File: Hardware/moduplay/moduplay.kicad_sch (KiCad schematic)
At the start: 11 parts, among them SW1 Left, SW10 Power_Switch, SW2 Up, SW3 Right, SW4 Down, SW5 X, SW6 Y, SW7 B, SW8 A, SW9 Menu

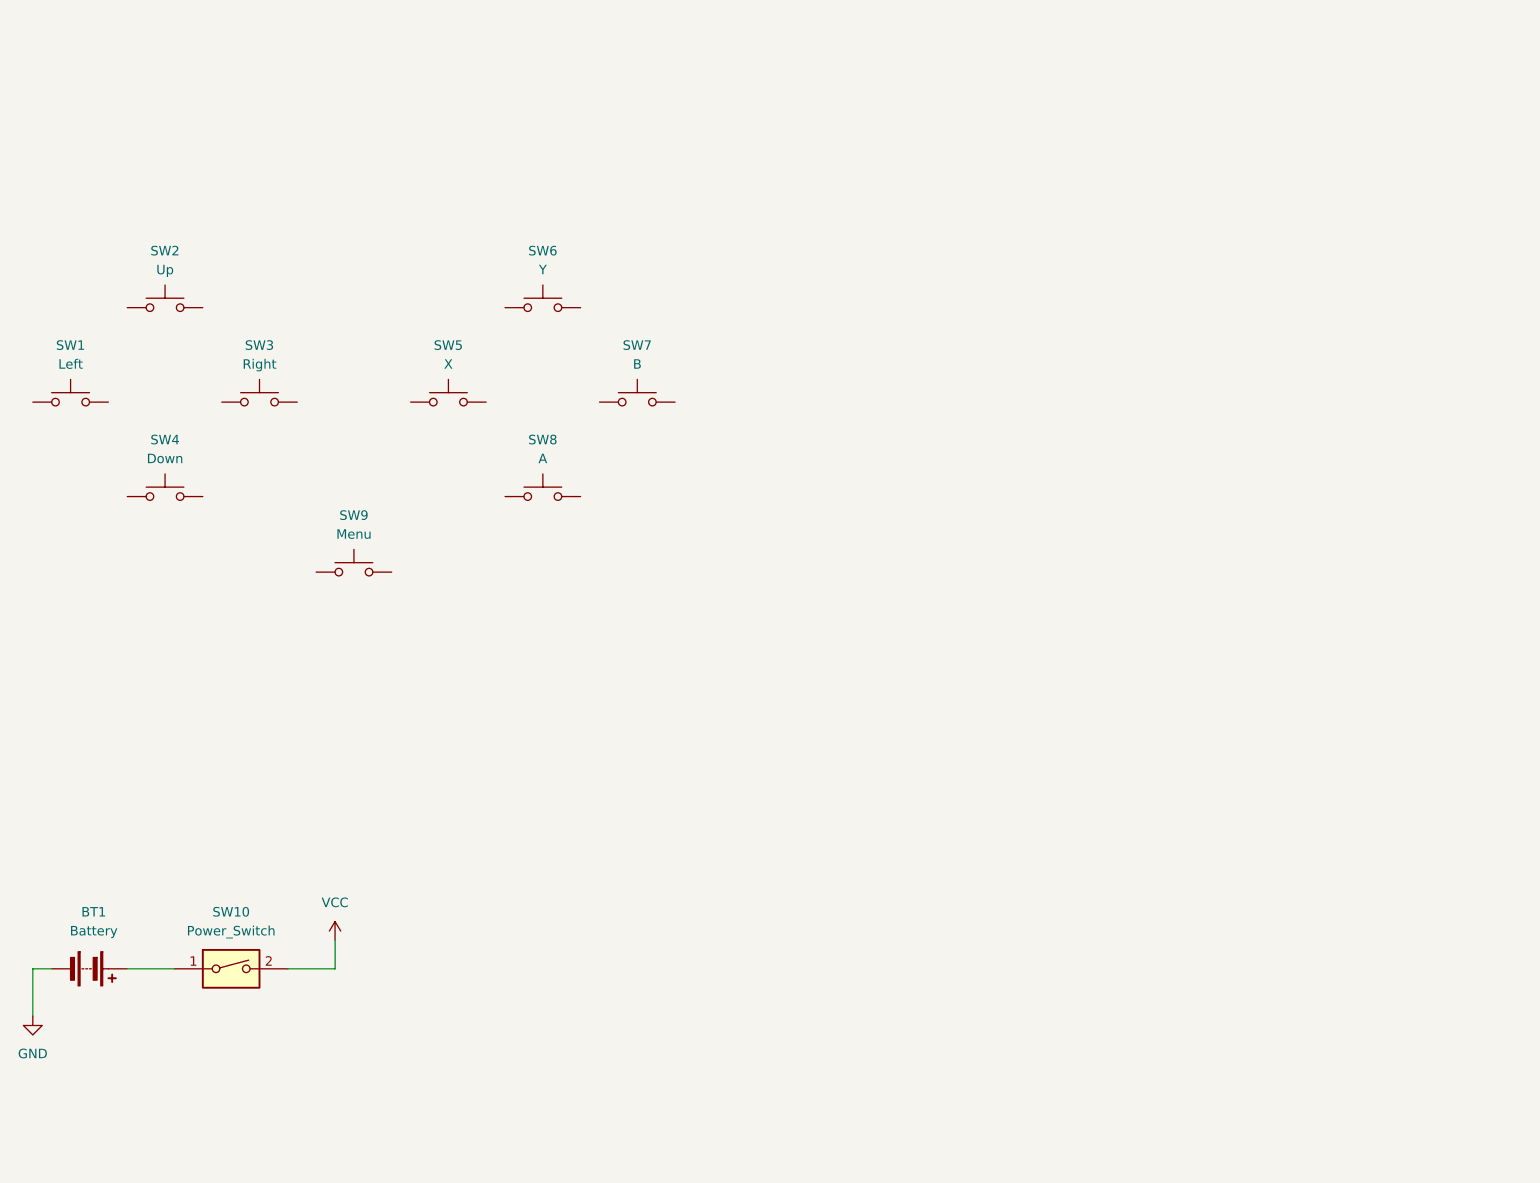
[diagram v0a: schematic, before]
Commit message: Finish scheme
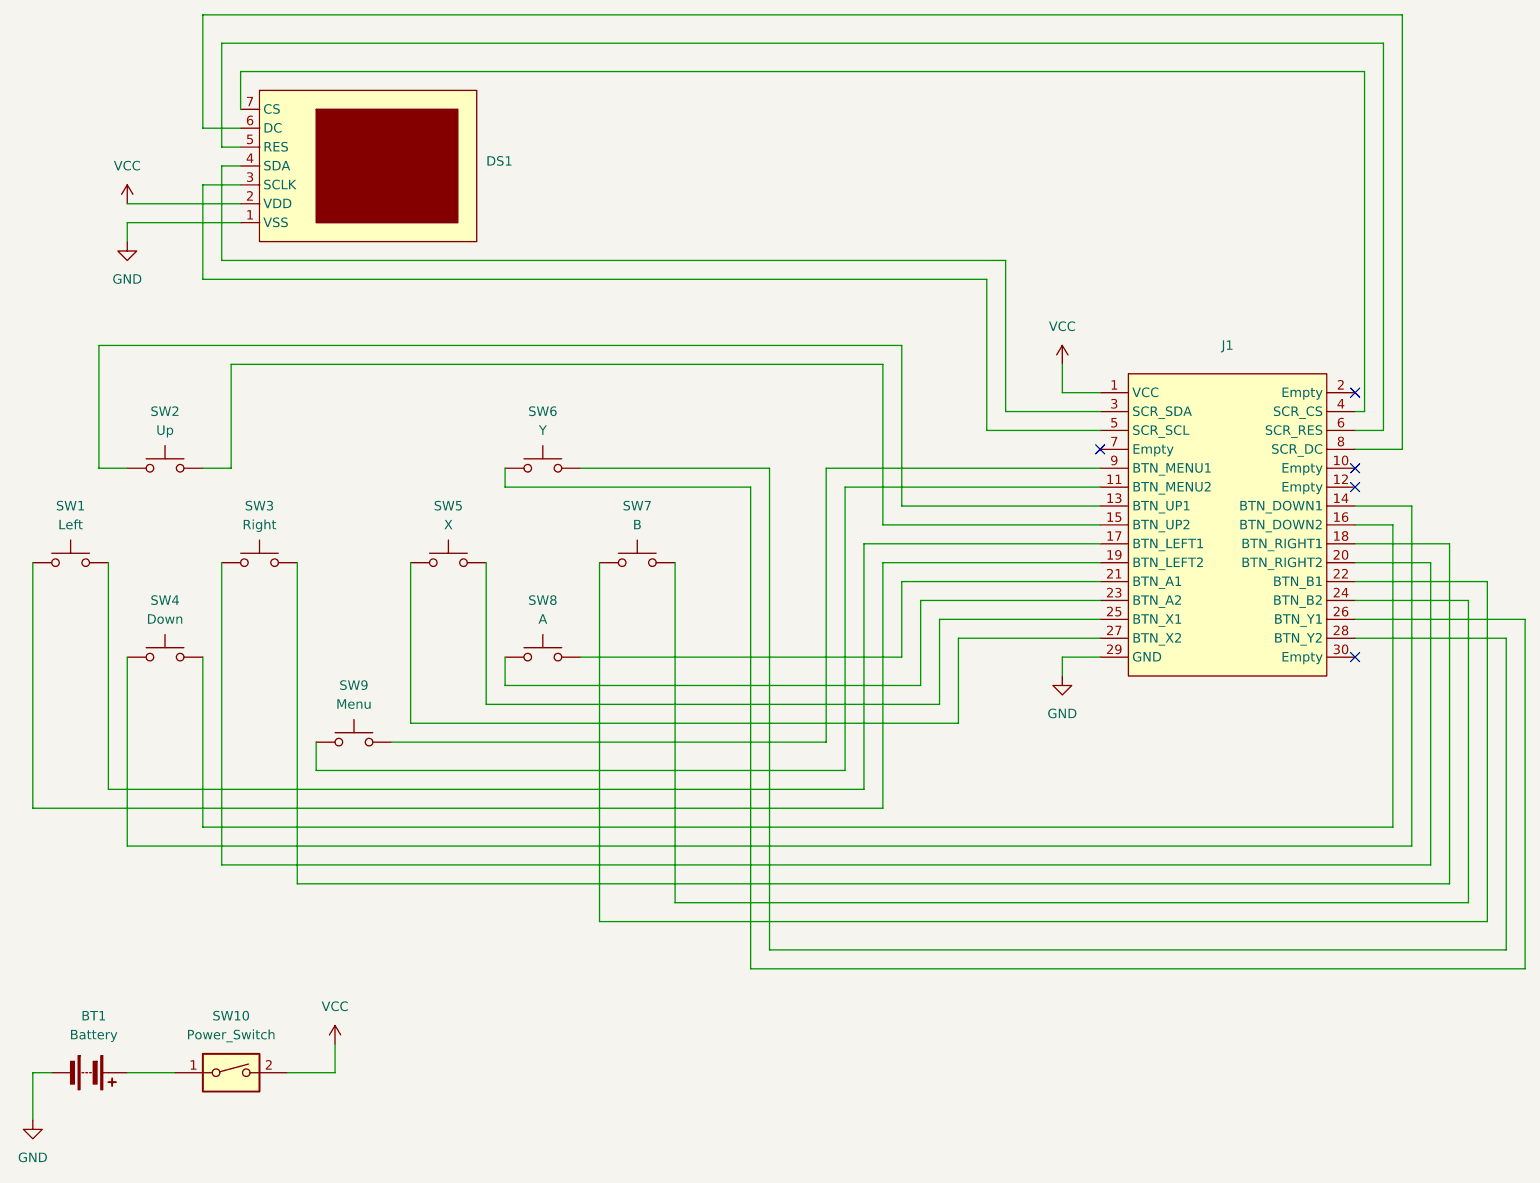
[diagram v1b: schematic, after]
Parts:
- added DS1: ~, symbol local:OLED12864_SPI_SSD1309
- added J1: ~, symbol local:Edge_Connector
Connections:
- net GND: now also DS1.1 (VSS), J1.29 (GND)
- net VCC: now also DS1.2 (VDD), J1.1 (VCC)
- net at SW3.1: now also J1.20 (BTN_RIGHT2)
- net at SW3.2: now also J1.18 (BTN_RIGHT1)
- net at SW6.1: now also J1.26 (BTN_Y1)
- net at SW6.2: now also J1.28 (BTN_Y2)
- net at SW9.1: now also J1.11 (BTN_MENU2)
- net at SW9.2: now also J1.9 (BTN_MENU1)
- net at SW2.1: now also J1.13 (BTN_UP1)
- net at SW2.2: now also J1.15 (BTN_UP2)
- net at SW1.1: now also J1.19 (BTN_LEFT2)
- net at SW1.2: now also J1.17 (BTN_LEFT1)
- net at SW8.1: now also J1.23 (BTN_A2)
- net at SW8.2: now also J1.21 (BTN_A1)
- net at SW5.1: now also J1.27 (BTN_X2)
- net at SW5.2: now also J1.25 (BTN_X1)
- net at SW4.1: now also J1.14 (BTN_DOWN1)
- net at SW4.2: now also J1.16 (BTN_DOWN2)
- net at SW7.1: now also J1.22 (BTN_B1)
- net at SW7.2: now also J1.24 (BTN_B2)
- new net: DS1.4 (SDA), J1.3 (SCR_SDA)
- new net: DS1.7 (CS), J1.4 (SCR_CS)
- new net: DS1.3 (SCLK), J1.5 (SCR_SCL)
- new net: DS1.5 (RES), J1.6 (SCR_RES)
- new net: DS1.6 (DC), J1.8 (SCR_DC)
- no-connect marks 0 -> 5
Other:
- title: (none) -> ModuPlay main board
- moved on the sheet: BT1, SW1, SW10, SW2, SW3, SW4, SW5, SW6, SW7, SW8, SW9
